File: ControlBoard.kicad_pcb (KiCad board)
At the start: 2 copper layers, 80 x 60 mm, 41 parts, among them J1 Conn_02x07_Odd_Even, J2 Conn_02x07_Odd_Even, J4 Conn_02x05_Odd_Even, J6 Conn_01x02_MountingPin, U1 STM32G473RCTx, U2 AT24CS02-XHM, U3 ICM-42668-P, U4 RT9013-33GB, U6 TLE9251VSJ

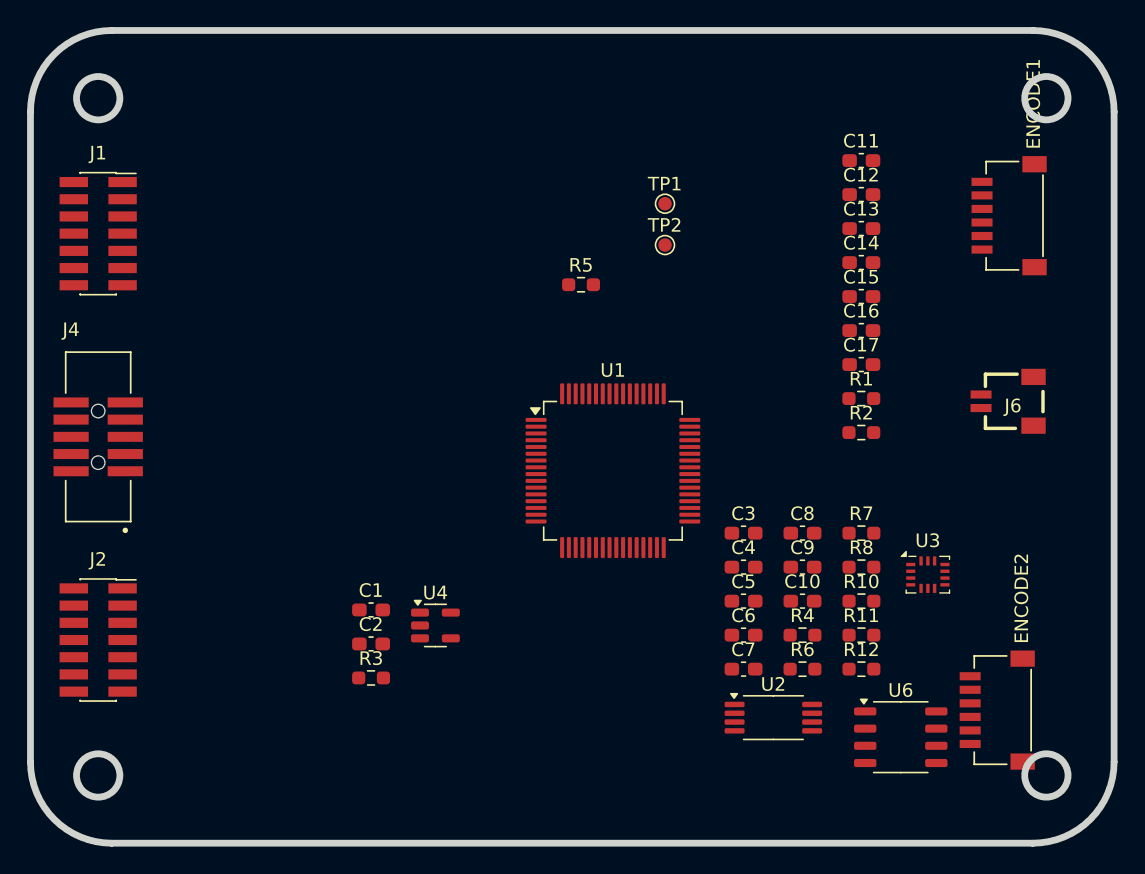
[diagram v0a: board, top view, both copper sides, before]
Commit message: PCB初布局
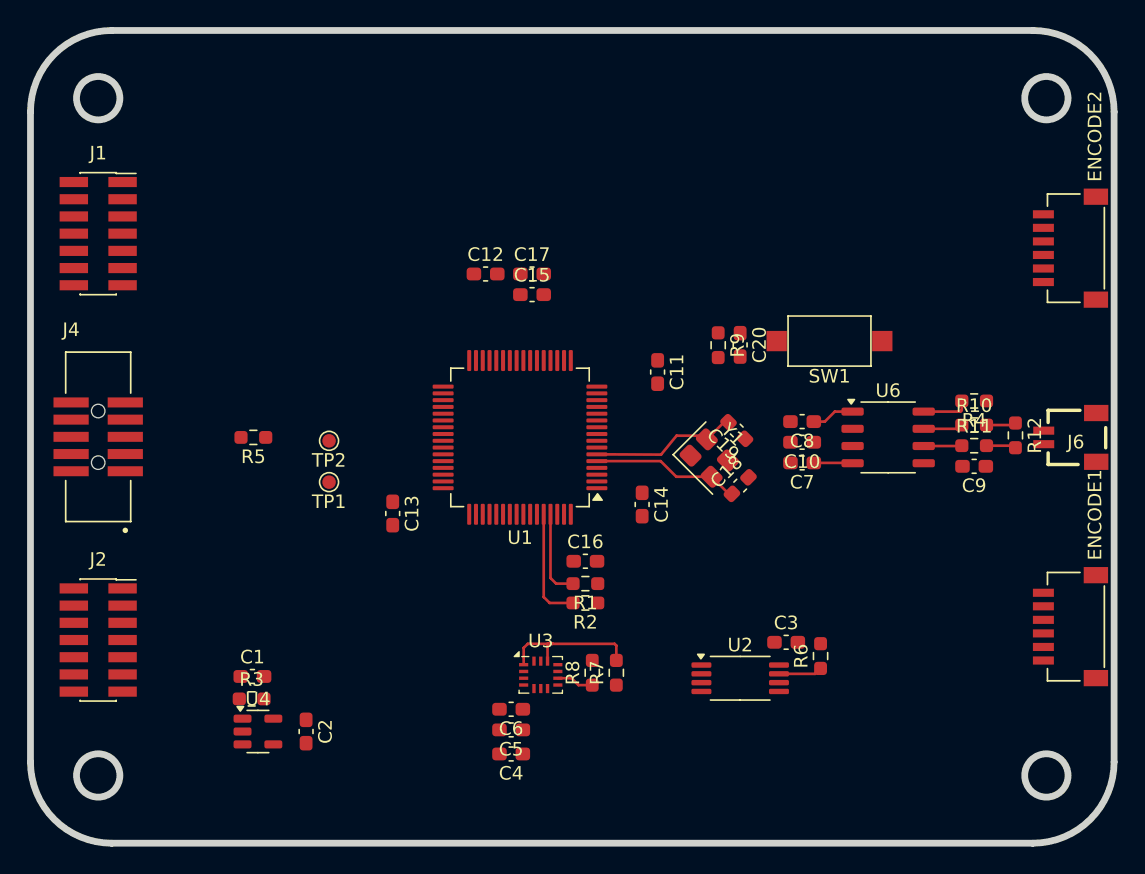
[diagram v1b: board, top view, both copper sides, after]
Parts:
- added C18: 22pF, Capacitor_SMD:C_0603_1608Metric_Pad1.08x0.95mm_HandSolder, F.Cu at (120.4, 85.6)
- added C19: 22pF, Capacitor_SMD:C_0603_1608Metric_Pad1.08x0.95mm_HandSolder, F.Cu at (120.1, 81.5)
- added C20: 0.1uF, Capacitor_SMD:C_0603_1608Metric_Pad1.08x0.95mm_HandSolder, F.Cu at (120.4, 75.2)
- added R9: 10K, Resistor_SMD:R_0603_1608Metric_Pad0.98x0.95mm_HandSolder, F.Cu at (118.8, 75.2)
- added SW1: SW_Push, Button_Switch_SMD:SW_SPST_CK_RS282G05A3, F.Cu at (127.0, 74.9)
- added Y1: 12MHz, Crystal:Crystal_SMD_3225-4Pin_3.2x2.5mm, F.Cu at (118.1, 83.6)
- moved C13 40.5 mm to (94.7, 87.7), turned to -90 degrees
- moved ENCODE2 34.5 mm to (142.8, 68.1)
- moved TP1 32.2 mm to (90.0, 85.3), turned to 180 degrees
- moved ENCODE1 30.7 mm to (142.8, 96.0)
- moved U3 29.5 mm to (105.7, 99.6)
- moved TP2 28.7 mm to (90.0, 82.3), turned to 180 degrees
- moved C12 28.4 mm to (101.6, 70.0)
- moved R5 26.7 mm to (84.5, 82.0), turned to 180 degrees
- moved C16 26.6 mm to (109.0, 91.2)
- moved C17 25.2 mm to (105.0, 70.0)
- moved R1 24.5 mm to (109.0, 92.8), turned to 180 degrees
- moved C15 24.3 mm to (105.0, 71.5)
- moved C14 24.1 mm to (113.2, 87.0), turned to -90 degrees
- moved R2 23.9 mm to (109.0, 94.3), turned to 180 degrees
- moved U6 22.2 mm to (131.3, 82.0)
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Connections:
- U1 pad 5: unconnected-(U1-PF0-Pad5) -> Net-(U1-PF0)
- U1 pad 6: unconnected-(U1-PF1-Pad6) -> Net-(U1-PF1)
- U1 pad 7: unconnected-(U1-PG10-Pad7) -> Net-(U1-PG10)
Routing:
- net Net-(U1-PF1): track 0.00 -> 11.0 mm
- net Net-(U3-AP_CS): track 0.00 -> 11.0 mm
- net Net-(U1-PF0): track 0.00 -> 11.0 mm
- net /MCU_Part/Peripheral/24C02_SDA: track 0.00 -> 8.45 mm
- net /MCU_Part/Peripheral/24C02_SCL: track 0.00 -> 6.54 mm
- net Net-(U6-STB): track 0.00 -> 3.54 mm
- net Net-(U2-WP): track 0.00 -> 3.24 mm
- net /MCU_Part/Peripheral/PB6_FDCAN2_TX: track 0.00 -> 3.17 mm
- net Net-(U6-CAN_H): track 0.00 -> 2.93 mm
- net /MCU_Part/Peripheral/PB11_FDCAN2_RX: track 0.00 -> 2.87 mm
- net Net-(U6-CAN_L): track 0.00 -> 2.82 mm
- net Net-(U3-INT2/FSYNC/CLKIN): track 0.00 -> 2.75 mm
- net /CAN_L: track 0.00 -> 2.20 mm
- net /CAN_H: track 0.00 -> 2.20 mm
